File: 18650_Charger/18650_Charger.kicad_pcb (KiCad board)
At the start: 2 copper layers, 16.6 x 14 mm, 12 parts, among them J1 IN_5V, J2 IN_0V, J3 BAT_5V, J4 BAT_0V, U1 TP4056

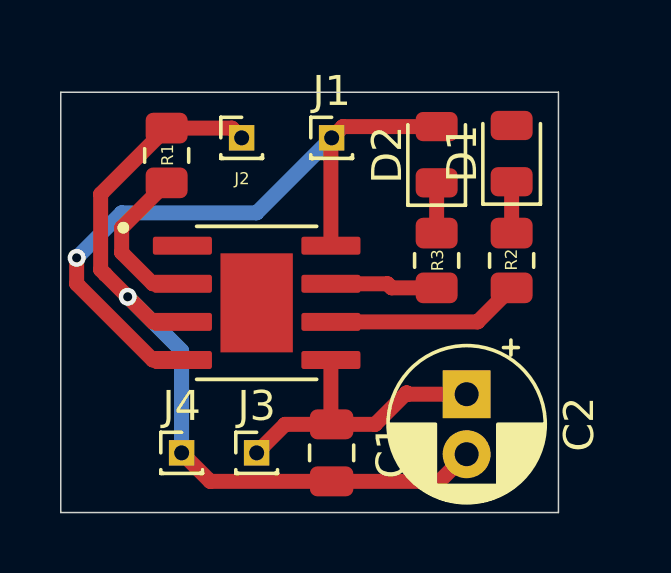
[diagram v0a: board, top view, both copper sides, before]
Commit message: V3
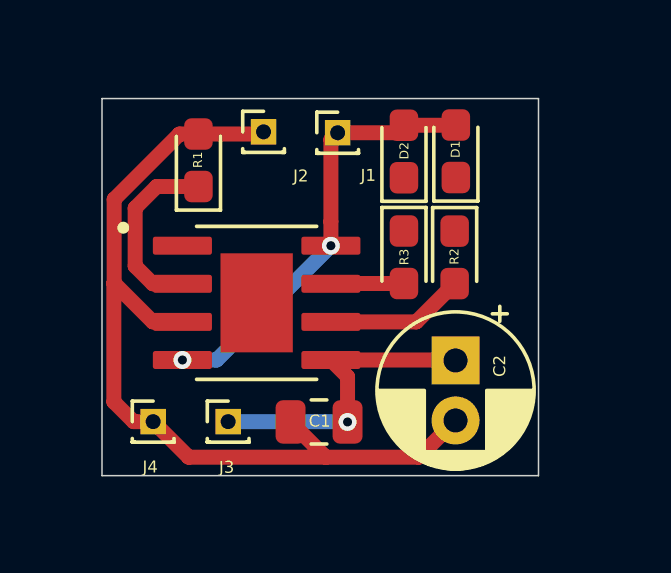
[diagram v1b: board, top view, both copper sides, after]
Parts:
- D1, D2: footprint LED_SMD:LED_0805_2012Metric -> LED_SMD:LED_0603_1608Metric_Pad1.05x0.95mm_HandSolder
- R1, R2, R3: footprint Resistor_SMD:R_0805_2012Metric -> LED_SMD:LED_0603_1608Metric_Pad1.05x0.95mm_HandSolder
- moved R2 1.90 mm to (134.6, 63.0)
- moved D1 1.86 mm to (134.6, 59.4)
- moved J3 1.41 mm to (127.0, 68.5)
- moved J4 1.41 mm to (124.5, 68.5)
- moved C2 1.18 mm to (134.6, 66.4)
- moved C1 1.11 mm to (130.1, 68.5), turned to 180 degrees
- moved D2 1.10 mm to (132.9, 59.5)
- moved R3 1.10 mm to (132.9, 63.0)
- moved R1 1.07 mm to (126.1, 59.7)
- moved J2 0.76 mm to (128.2, 58.8)
- moved J1 0.26 mm to (130.7, 58.8)
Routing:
- net Net-(D1-A): track 22.9 -> 14.4 mm, vias 1 -> 2
- net Net-(U1-~{STDBY}): track 6.50 -> 4.65 mm
- net Net-(D1-K): track 1.71 -> 0.00 mm
- net Net-(D2-K): track 1.67 -> 0.00 mm
- net 0: track 28.3 -> 29.8 mm, vias 1 -> 0
- net Net-(U1-~{CHRG}): track 3.58 -> 2.44 mm
- net Net-(U1-PROG): track 5.40 -> 6.16 mm
- net Net-(J3-Pin_1): track 10.0 -> 10.4 mm, vias 0 -> 1
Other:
- board size 16.6 x 14 mm -> 14.6 x 12.6 mm

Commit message: V1
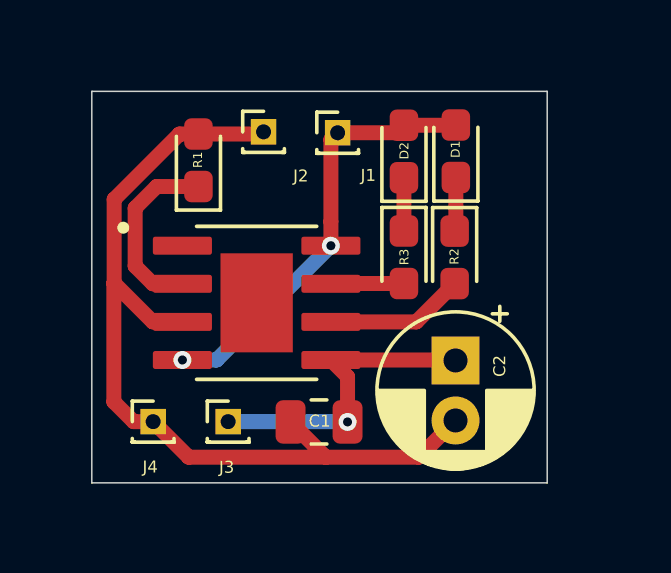
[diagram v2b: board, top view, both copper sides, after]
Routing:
- net Net-(D1-K): track 0.00 -> 1.80 mm
- net Net-(D2-K): track 0.00 -> 1.77 mm
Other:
- board size 14.6 x 12.6 mm -> 15.2 x 13 mm
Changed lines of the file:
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@@
 	)
 	(gr_rect
-		(start 122.845 57.69)
-		(end 137.395 70.26)
+		(start 122.505 57.45)
+		(end 137.685 70.5)
 		(stroke
 			(width 0.05)
@@
 	)
 	(segment
+		(start 134.64 60.3225)
+		(end 134.64 62.06875)
+		(width 0.5)
+		(layer "F.Cu")
+		(net 5)
+	)
+	(segment
+		(start 134.64 62.06875)
+		(end 134.6 62.10875)
+		(width 0.5)
+		(layer "F.Cu")
+		(net 5)
+	)
+	(segment
+		(start 132.91 60.33)
+		(end 132.91 62.105)
+		(width 0.5)
+		(layer "F.Cu")
+		(net 6)
+	)
+	(segment
